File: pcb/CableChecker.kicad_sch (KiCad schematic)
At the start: 11 parts, among them J1 AudioJack3_SwitchTR, J2 NC3MAAH, J3 NC3FAAH, SW1 RotaryEncoder_Switch_MP, U1 ES8388

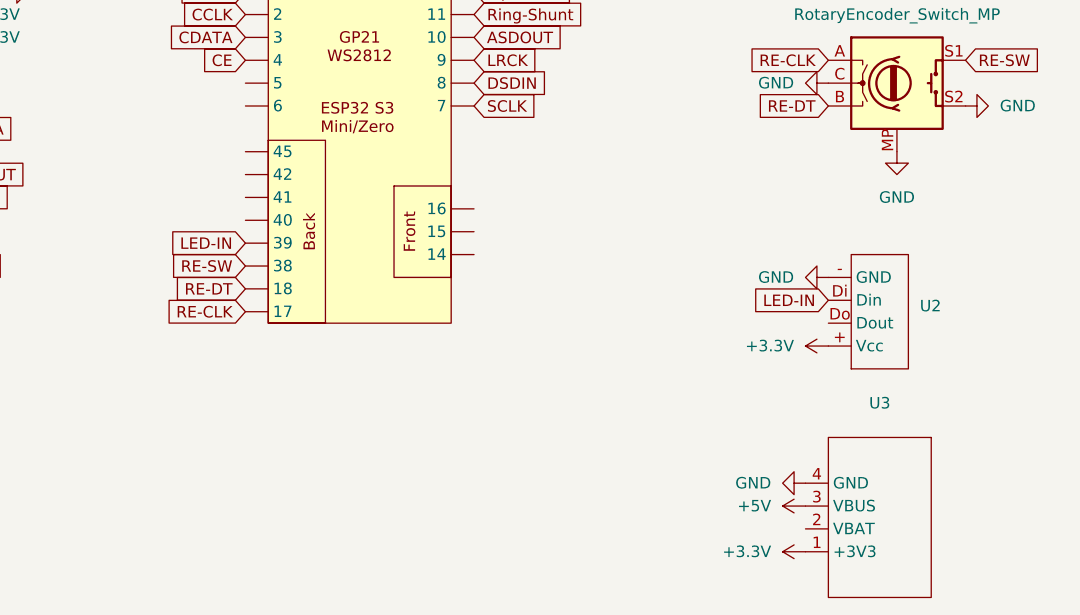
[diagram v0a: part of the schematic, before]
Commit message: added adf
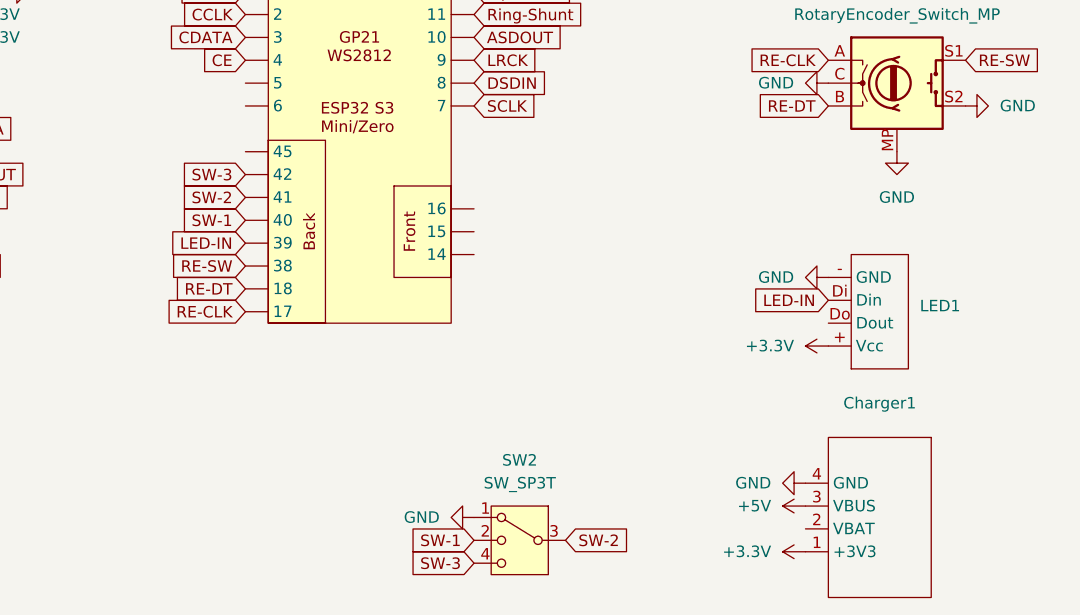
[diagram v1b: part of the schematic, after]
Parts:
- added SW2: SW_SP3T, easyeda2kicad:SW-TH_SK13D07VG5, symbol Switch:SW_SP3T
- LED1: renamed from U2; footprint (none) -> LED_SMD:GlowbitL_LED_Strip_1x8
- renumbered U3 to Charger1
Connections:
- net GND: now also SW2.1
- new net SW-1: ESP32_S1. (14), SW2.2
- new net SW-2: ESP32_S1. (14), SW2.3
- new net SW-3: ESP32_S1. (14), SW2.4
